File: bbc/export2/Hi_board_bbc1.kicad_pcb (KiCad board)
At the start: 2 copper layers, 55 x 55.4 mm, 15 parts, among them J1 sw-latchboard, J2 led-latchboard, J3 GLVMP, SW1 BSPD_RESET, SW2 IMD_RESET, SW3 BMS_RESET

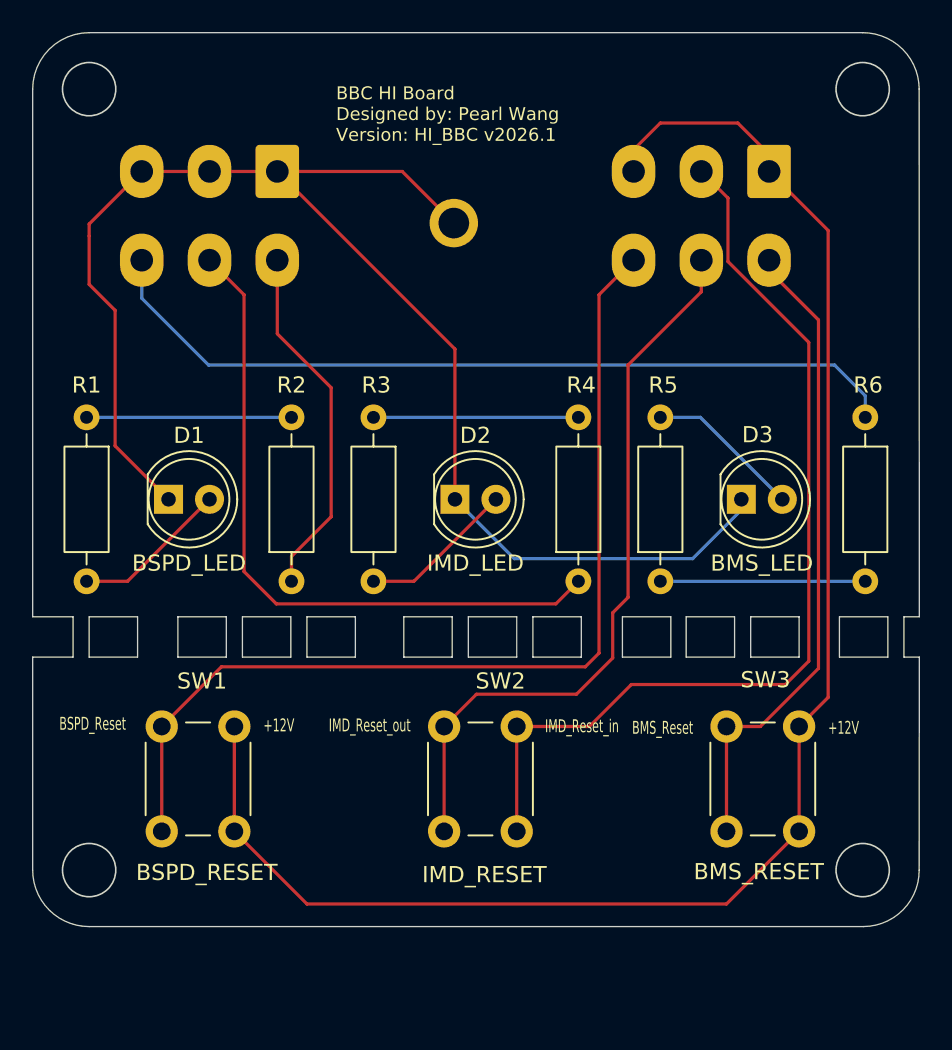
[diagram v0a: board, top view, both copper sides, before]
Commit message: Add files via upload
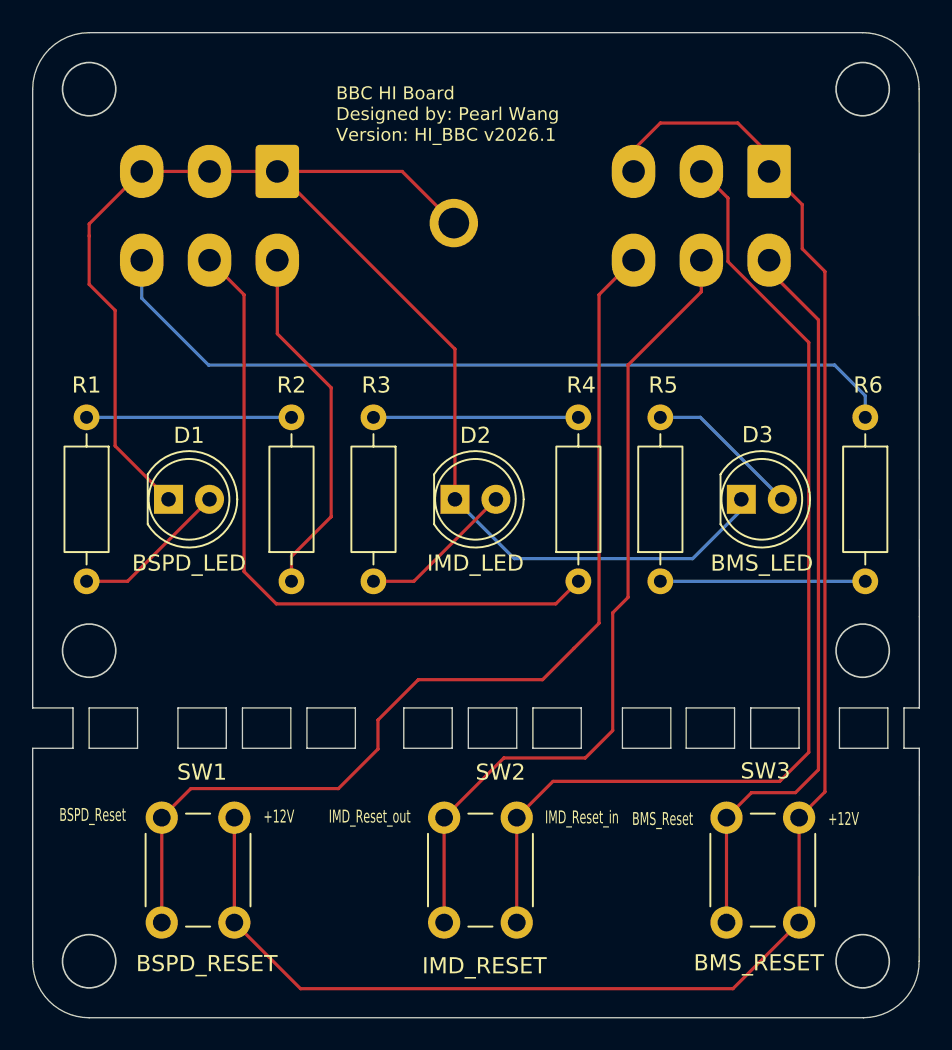
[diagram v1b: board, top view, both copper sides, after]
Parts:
- moved SW1 5.65 mm to (121.5, 148.2)
- moved SW2 5.65 mm to (139.0, 148.2)
- moved SW3 5.65 mm to (156.5, 148.2)
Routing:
- net BMS_RESET: track 40.3 -> 46.3 mm
- net Net-(J1-Pin_2): track 59.4 -> 65.0 mm
- net +12V: track 100.7 -> 105.8 mm
- net IMD_RESET: track 45.6 -> 50.6 mm
- net BSPD_RESET: track 60.7 -> 63.0 mm
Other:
- board size 55 x 55.4 mm -> 55 x 61.1 mm
